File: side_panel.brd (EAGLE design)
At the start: 81.7 x 112 mm, 35 parts

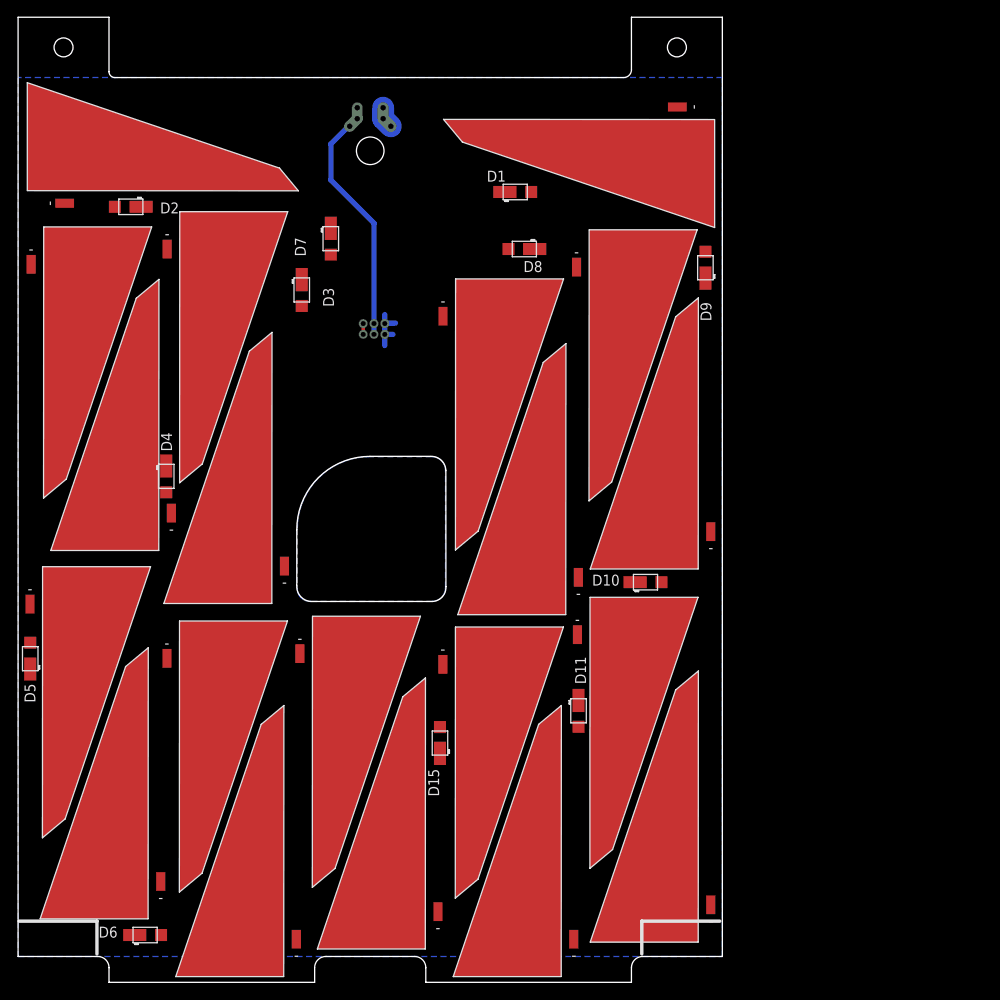
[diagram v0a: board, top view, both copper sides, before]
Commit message: Finished solar panel layout
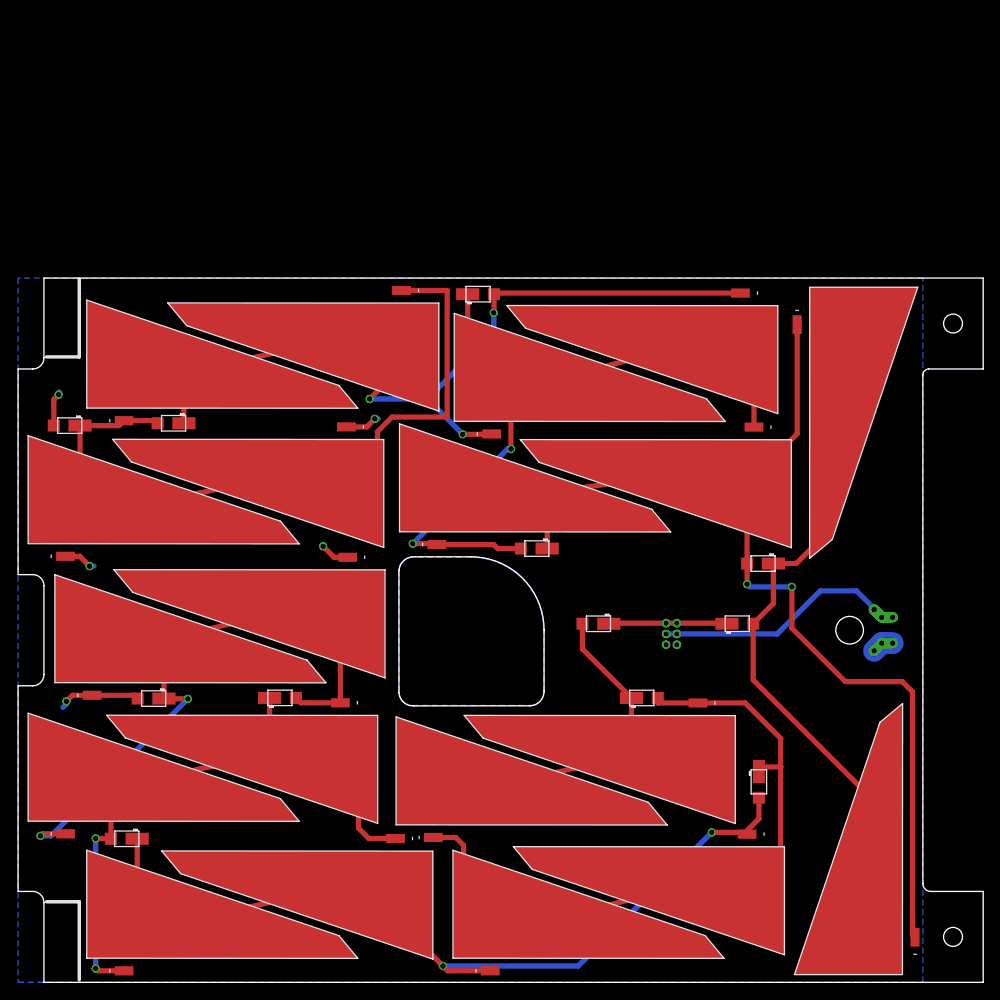
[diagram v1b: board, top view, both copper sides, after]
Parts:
- removed D15: SB_DIODE, phonesat:SB_DIODE
- added D12: SB_DIODE, phonesat:SB_DIODE
- moved SL2 96.2 mm to (102.5, 8.23), turned to 180 degrees
- moved U$2 85.8 mm to (101.5, 39.4), turned to 180 degrees
- moved U$4 85.8 mm to (101.5, 42.4), turned to 0 degrees
- moved SL1 85.7 mm to (92.0, 73.3), turned to 0 degrees
- moved D2 84.2 mm to (86.5, 48.6)
- moved SL5 77.8 mm to (80.8, 78.4), turned to 270 degrees
- moved D10 67.2 mm to (12.6, 16.7), turned to 180 degrees
- moved SL3 66.4 mm to (82.4, 62.8), turned to 270 degrees
- moved SL13 66.2 mm to (81.6, 15.6), turned to 270 degrees
- moved SL16 64.1 mm to (15.3, 2.93), turned to 90 degrees
- moved D9 60.0 mm to (86.0, 23.3), turned to 270 degrees
- moved D6 59.8 mm to (5.99, 64.6), turned to 180 degrees
- moved SL14 56.4 mm to (57.8, 2.93), turned to 90 degrees
- moved D1 56.3 mm to (83.5, 41.6)
- moved SL18 55.5 mm to (8.50, 18.8), turned to 90 degrees
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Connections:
- net GND: now also D12.POS; no longer D15.POS
- net N$6: now also D12.NEG; no longer D15.NEG
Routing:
- net N$45: track 0.00 -> 148.7 mm, vias 0 -> 2
- net N$39: track 0.00 -> 121.1 mm, vias 0 -> 3
- net N$3: track 0.00 -> 116.1 mm, vias 0 -> 2
- net N$6: track 0.00 -> 100.1 mm, vias 0 -> 2
- net N$4: track 0.00 -> 98.8 mm, vias 0 -> 2
- net N$37: track 0.00 -> 98.1 mm, vias 0 -> 2
- net N$50: track 0.30 -> 94.5 mm
- net N$9: track 0.00 -> 86.7 mm
- net N$2: track 0.00 -> 85.4 mm
- net N$8: track 0.00 -> 60.7 mm
- net GND: track 2.53 -> 27.8 mm, vias 0 -> 5
- net V_SOLAR: track 1.27 -> 13.8 mm
- net N$7: track 3.60 -> 0.00 mm
- net N$5: track 1.30 -> 0.00 mm
- net N$1: track 0.90 -> 0.00 mm
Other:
- board size 81.7 x 112 mm -> 112 x 81.7 mm
- board text added: "Side Solar Panel V1.1"
